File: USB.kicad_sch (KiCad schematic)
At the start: 1 part, among them U2 Compute_Module_4_Functional

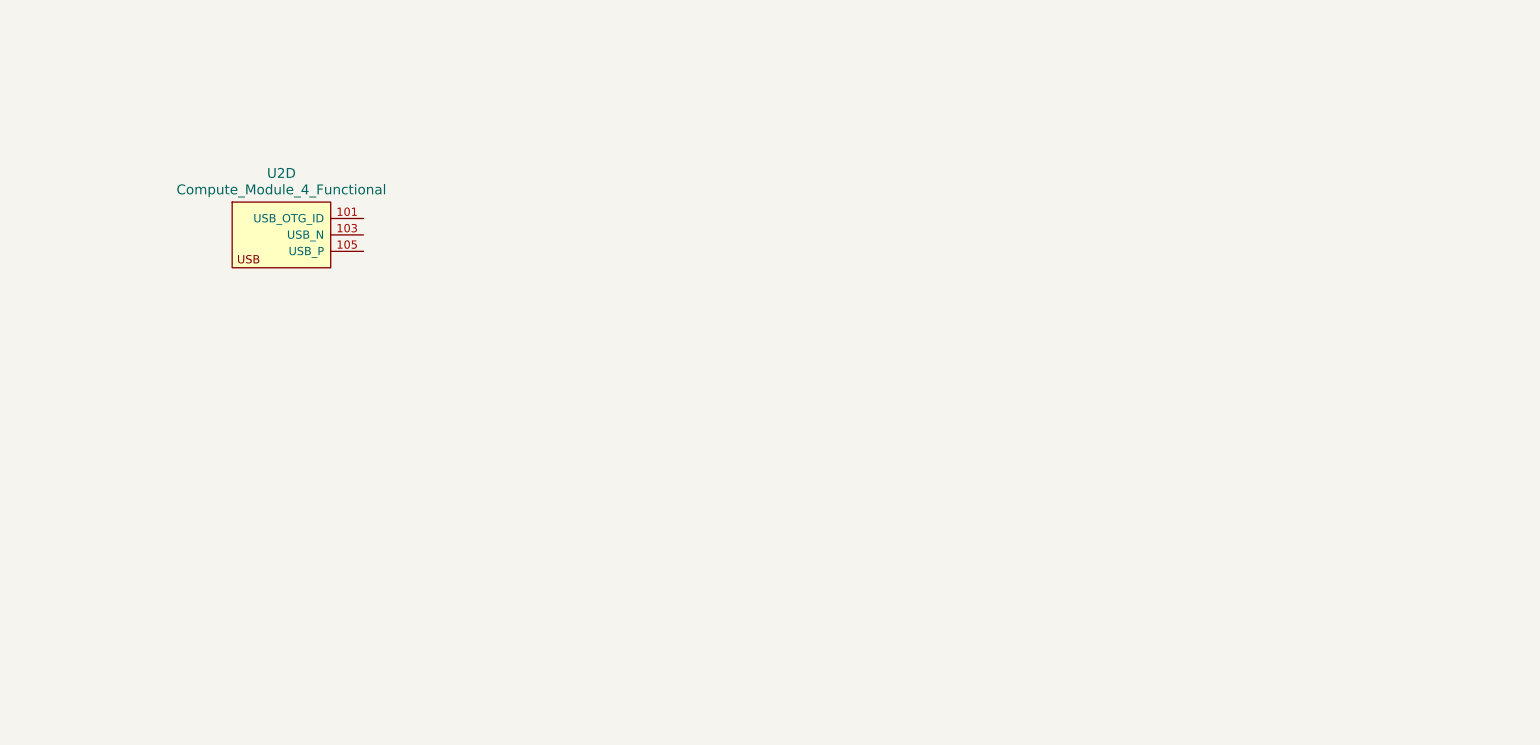
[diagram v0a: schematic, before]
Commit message: added display things + others
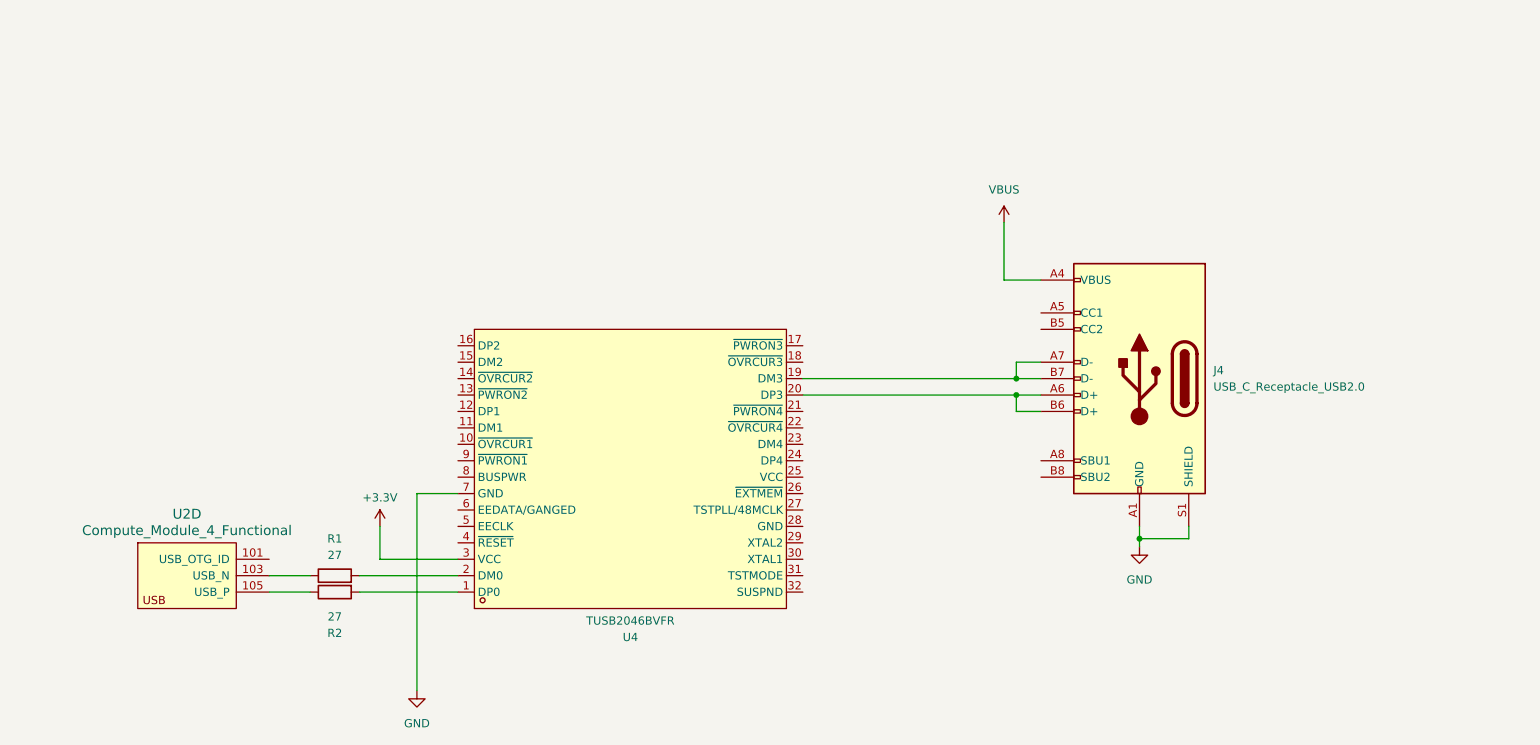
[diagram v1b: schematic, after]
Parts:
- added J4: USB_C_Receptacle_USB2.0, symbol Connector:USB_C_Receptacle_USB2.0
- added R1, R2: 27, symbol Device:R
- added U4: TUSB2046BVFR, easyeda2kicad:LQFP-32_L7.0-W7.0-P0.80-LS9.0-TL, symbol easyeda2kicad:TUSB2046BVFR
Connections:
- net at U2.103 (USB_N): now also R1.1
- net at U2.105 (USB_P): now also R2.1
- new net: J4.A6 (D+), J4.B6 (D+), U4.20 (DP3)
- new net: J4.A7 (D-), J4.B7 (D-), U4.19 (DM3)
- new net: R1.2, U4.2 (DM0)
- new net: R2.2, U4.1 (DP0)
- new net +3.3V: U4.3 (VCC)
- new net GND: J4.A1 (GND), J4.A12 (GND), J4.B1 (GND), J4.B12 (GND), J4.S1 (SHIELD), U4.7 (GND)
- new net VBUS: J4.A4 (VBUS), J4.A9 (VBUS), J4.B4 (VBUS), J4.B9 (VBUS)
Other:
- moved on the sheet: U2D

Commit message: audio and display changes
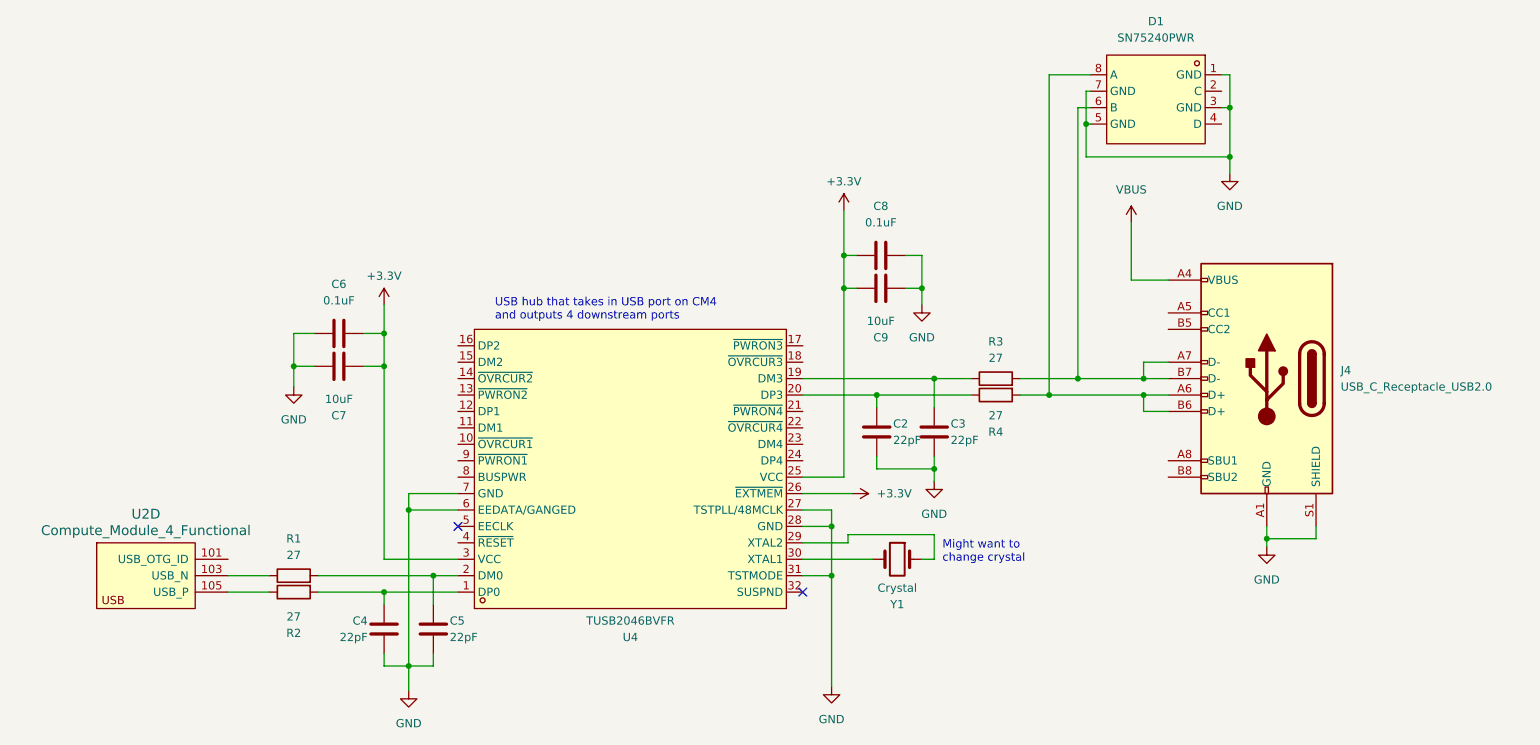
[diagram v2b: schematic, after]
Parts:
- added C2, C3, C4, C5: 22pF, symbol Device:C
- added C6, C8: 0.1uF, symbol Device:C
- added C7, C9: 10uF, symbol Device:C
- added D1: SN75240PWR, easyeda2kicad:TSSOP-8_L4.4-W3.0-P0.65-LS6.4-BL, symbol easyeda2kicad:SN75240PWR
- added R3, R4: 27, symbol Device:R
- added Y1: Crystal, symbol Device:Crystal
- J4: footprint (none) -> Connector_USB:USB_C_Receptacle_HRO_TYPE-C-31-M-12
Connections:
- net +3.3V: now also U4.25 (VCC), U4.26 (~{EXTMEM}), C6.2, C7.2, C8.1, C9.1
- net GND: now also U4.27 (TSTPLL/48MCLK), U4.28 (GND), U4.31 (TSTMODE), U4.6 (EEDATA/GANGED), C2.2, C3.2, C4.2, C5.2, C6.1, C7.1, C8.2, C9.2, D1.1 (GND), D1.3 (GND), D1.5 (GND), D1.7 (GND)
- net at J4.A6 (D+), J4.B6 (D+): now also D1.8 (A), R4.2; no longer U4.20 (DP3)
- net at J4.A7 (D-), J4.B7 (D-): now also D1.6 (B), R3.2; no longer U4.19 (DM3)
- net at R1.2, U4.2 (DM0): now also C5.1
- net at R2.2, U4.1 (DP0): now also C4.1
- net at U4.29 (XTAL2): now also Y1.1
- net at U4.30 (XTAL1): now also Y1.2
- new net: C3.1, R3.1, U4.19 (DM3)
- new net: C2.1, R4.1, U4.20 (DP3)
- no-connect marks 0 -> 2
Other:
- note added: "Might want to change crystal"
- note added: "USB hub that takes in USB port on CM4 and outputs 4 downstream ports"
- moved on the sheet: J4, R1, R2, U2D
